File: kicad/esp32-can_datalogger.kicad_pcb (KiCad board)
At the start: 2 copper layers, 60 x 40 mm, 51 parts, among them J1 USB_C_Receptacle_USB2.0_16P, J2 USB_C_Receptacle_USB2.0_16P, J3 USB_C_Receptacle_USB2.0_16P, J4 USB_C_Receptacle_USB2.0_16P, J5 Conn_01x04_Socket, J6 Conn_Coaxial, J7 MicroSD, SW1 SW_Push, SW2 SW_Push, SW3 SW_Push, SW4 SW_Push, U2 PA1616D, U3 PI4ULS3V204LEX, U5 TJA1051T, U6 TJA1051T, U7 ICM-20948

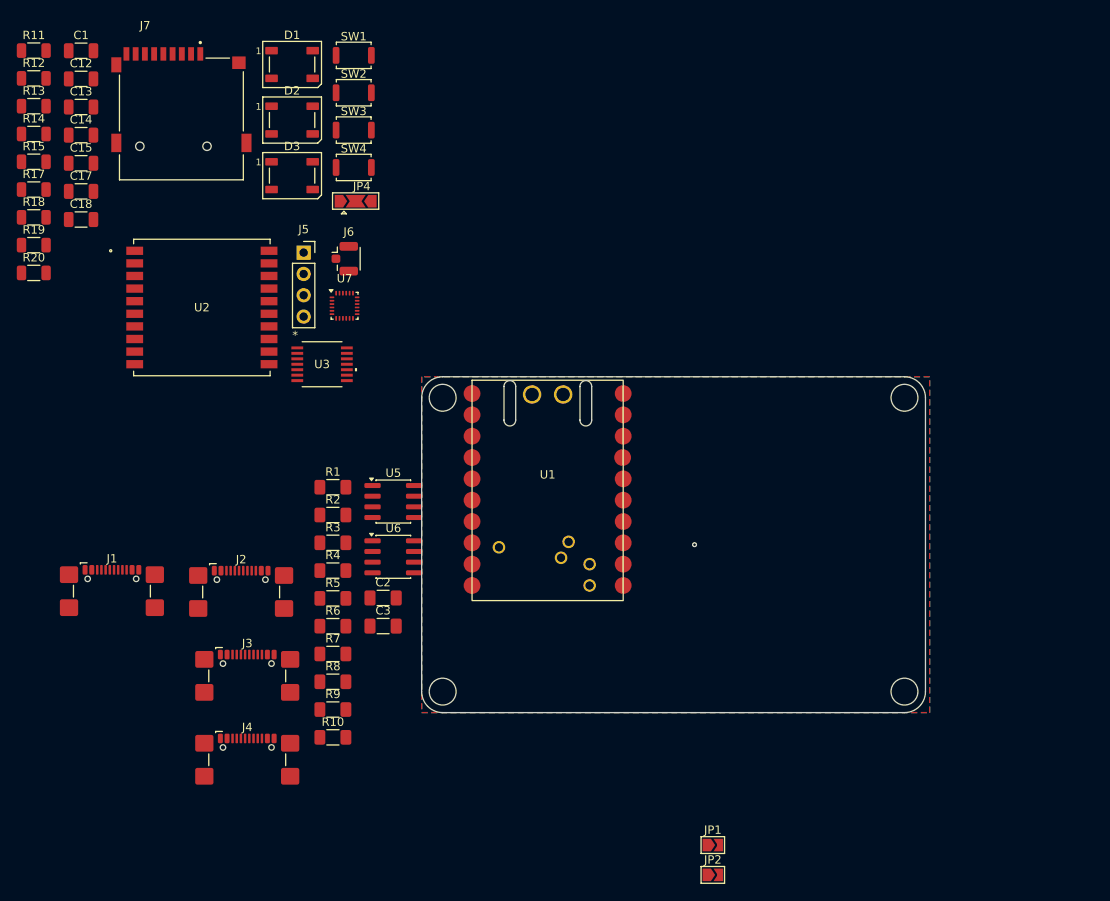
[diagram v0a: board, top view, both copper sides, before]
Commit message: pcb updates
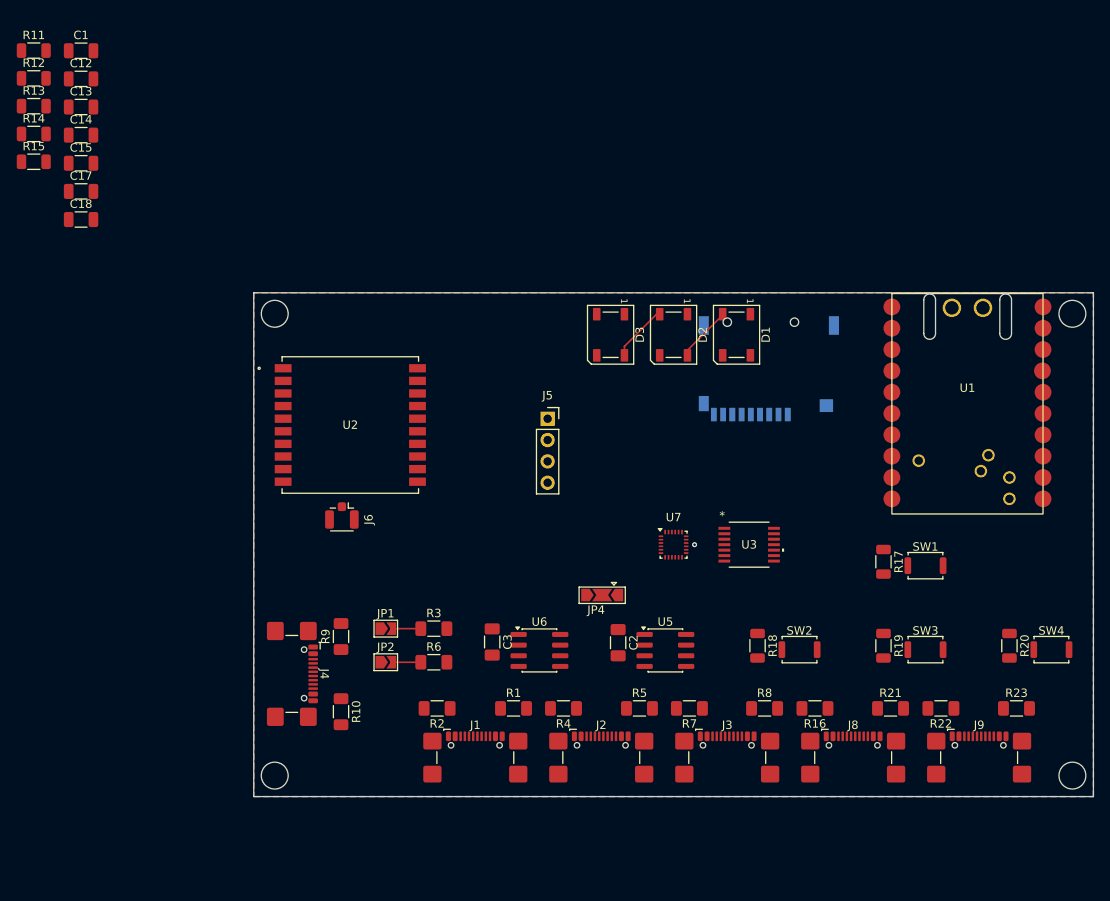
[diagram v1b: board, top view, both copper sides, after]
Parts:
- added J8: USB_C_Receptacle_USB2.0_16P, Connector_USB:USB_C_Receptacle_GCT_USB4110, F.Cu at (121.4, 126.5)
- added J9: USB_C_Receptacle_USB2.0_16P, Connector_USB:USB_C_Receptacle_GCT_USB4110, F.Cu at (136.4, 126.5)
- added R16: 5K1, Resistor_SMD:R_1206_3216Metric_Pad1.30x1.75mm_HandSolder, F.Cu at (116.8, 119.5)
- added R21: 5K1, Resistor_SMD:R_1206_3216Metric_Pad1.30x1.75mm_HandSolder, F.Cu at (125.8, 119.5)
- added R22: 5K1, Resistor_SMD:R_1206_3216Metric_Pad1.30x1.75mm_HandSolder, F.Cu at (131.8, 119.5)
- added R23: 5K1, Resistor_SMD:R_1206_3216Metric_Pad1.30x1.75mm_HandSolder, F.Cu at (140.8, 119.5)
- J7: moved to B.Cu
- moved R20 124.4 mm to (140.0, 112.0), turned to -90 degrees
- moved R19 111.9 mm to (125.0, 112.0), turned to -90 degrees
- moved R17 110.5 mm to (125.0, 102.0), turned to -90 degrees
- moved SW4 101.0 mm to (145.0, 112.5)
- moved R18 100.2 mm to (110.0, 112.0), turned to -90 degrees
- moved SW3 92.0 mm to (130.0, 112.5)
- moved SW1 91.3 mm to (130.0, 102.5)
- moved SW2 85.0 mm to (115.0, 112.5)
- moved J7 75.2 mm to (111.3, 76.8)
- moved D1 61.9 mm to (107.5, 75.0), turned to -90 degrees
- moved J3 58.0 mm to (106.4, 126.5)
- moved JP4 55.3 mm to (91.5, 106.0), turned to 180 degrees
- moved U3 55.2 mm to (109.0, 100.0)
- moved D2 52.1 mm to (100.0, 75.0), turned to -90 degrees
- moved R8 51.5 mm to (110.8, 119.5)
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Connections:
- J3 pad A6: /CAN1H -> /CAN0H
- J3 pad A7: /CAN1L -> /CAN0L
- J3 pad B6: /CAN1H -> /CAN0H
- J3 pad B7: /CAN1L -> /CAN0L
- J4 pad A6: /CAN0H -> /CAN1H
- J4 pad A7: /CAN0L -> /CAN1L
- J4 pad B6: /CAN0H -> /CAN1H
- J4 pad B7: /CAN0L -> /CAN1L
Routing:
- net Net-(D2-DOUT): track 0.00 -> 6.86 mm
- net Net-(D1-DOUT): track 0.00 -> 6.64 mm
- net Net-(JP2-B): track 0.00 -> 3.45 mm
- net Net-(JP1-B): track 0.00 -> 3.45 mm
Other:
- board size 60 x 40 mm -> 100 x 60 mm
